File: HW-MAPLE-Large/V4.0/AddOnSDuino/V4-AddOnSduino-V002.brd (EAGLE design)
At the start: 31 x 22.1 mm, 5 parts

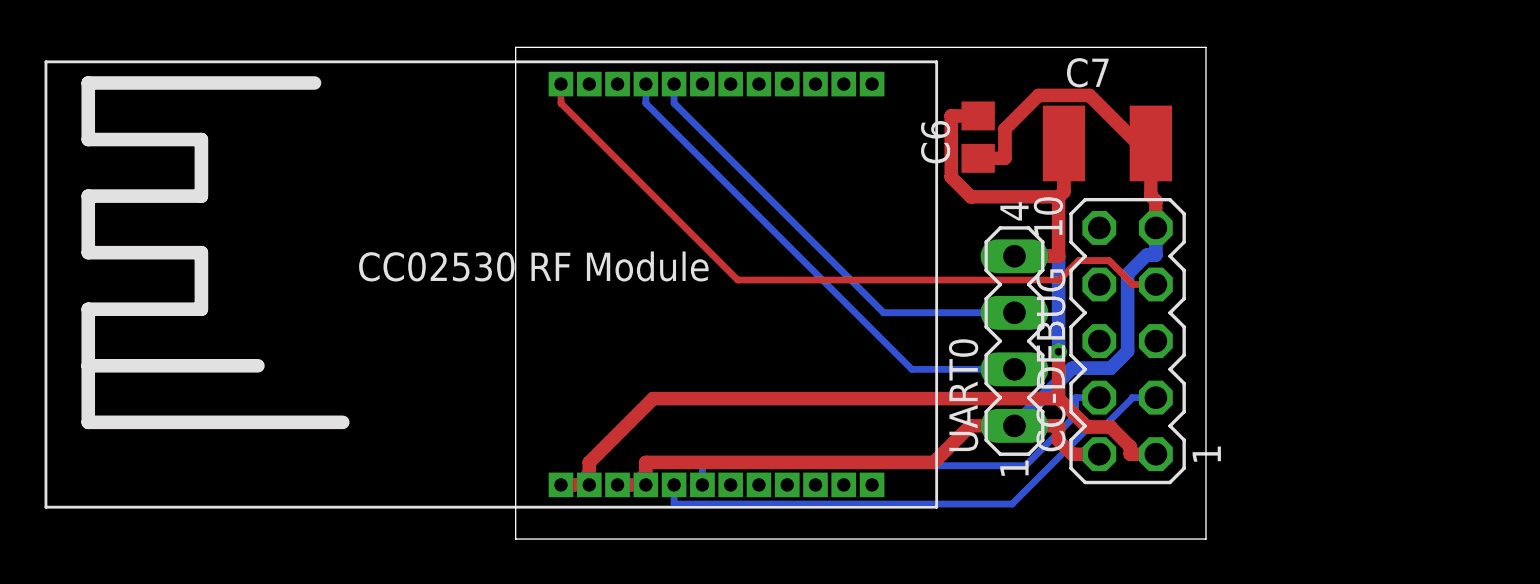
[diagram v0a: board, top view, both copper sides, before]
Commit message: V4 Test
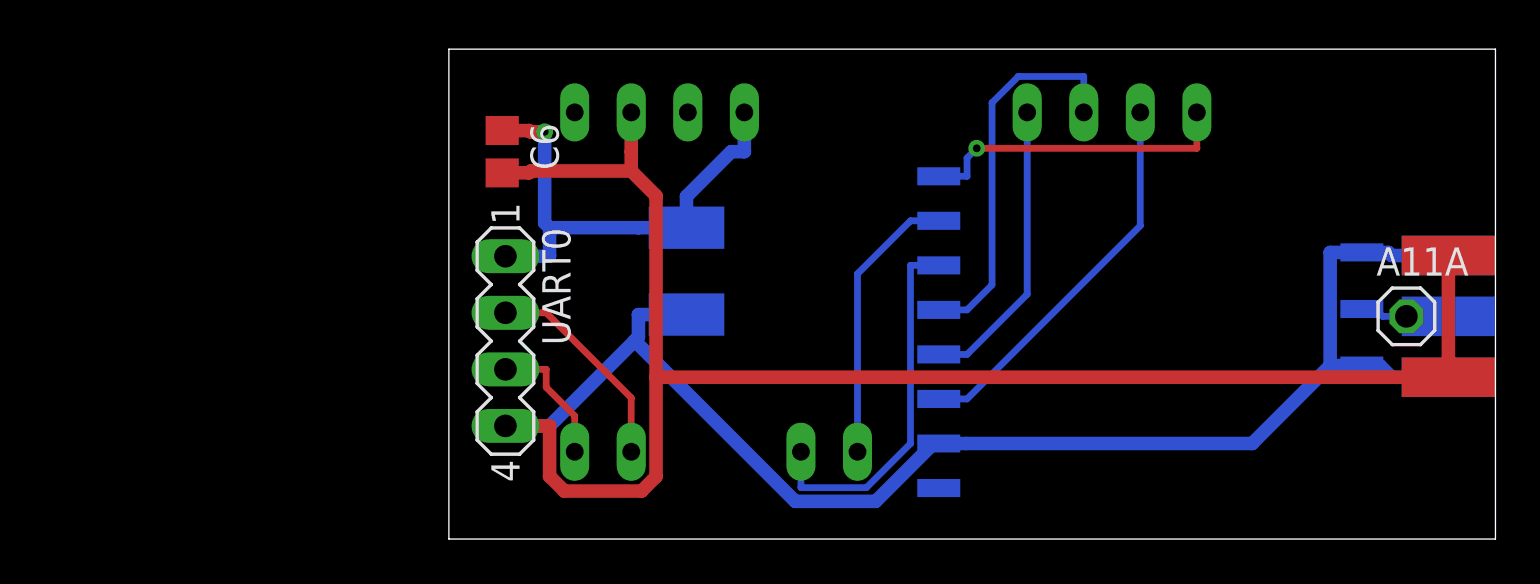
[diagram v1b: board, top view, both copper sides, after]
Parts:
- removed CC-DEBUG: (no value), con-lstb:MA05-2
- removed U$1: CC2530CC2530PA, zigbee:CC2530PA
- added A11A: (no value), pinhead:1X01
- added A11B: SMA, wireless:SMA
- added CC1101: CC1101_MODULE1SMD, CC1101:CC1101_MODULE1_SMD
- added U$2: MARTIN-PROMINI-CC1101, Arduino-clone:MARTIN-PRO-CC1101
- moved UART0 22.9 mm to (2.54, 8.89), turned to 270 degrees
- moved C6 21.4 mm to (2.40, 17.4), turned to 270 degrees
- moved C7 19.8 mm to (10.7, 12.0), flipped to the bottom, turned to 90 degrees
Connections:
- removed net BT: U$1.P$6
- removed net CS: CC-DEBUG.5
- removed net DC: CC-DEBUG.3, U$1.P$8
- removed net DD: CC-DEBUG.4, U$1.P$7
- removed net RST: CC-DEBUG.7, U$1.P$24
- removed net RX0: U$1.P$20, UART0.3
- removed net SCLK: CC-DEBUG.6
- removed net TX0: U$1.P$21, UART0.2
- new net +3V3: CC1101.VCC
- new net ANT1: A11A.1, A11B.1, CC1101.ANT
- new net CSN: CC1101.CSN, U$2.D10
- new net GDO0_D3: CC1101.GDO0, U$2.D3
- new net GDO2_D2: CC1101.GDO2, U$2.D2
- new net RX-MAPLE0: U$2.TX0, UART0.3
- new net SCK: CC1101.SCLK, U$2.D13
- new net TX-MAPLE0: U$2.RX1, UART0.2
- net GND: now also A11B.GND@1, A11B.GND@2, A11B.GND@3, A11B.GND@4, CC1101.GND@0, CC1101.GND@1, CC1101.GND@2, U$2.GND; no longer CC-DEBUG.1, U$1.P$11, U$1.P$12
- net MISO: now also CC1101.MISO, U$2.D12; no longer CC-DEBUG.10
- net MOSI: now also CC1101.MOSI, U$2.D11; no longer CC-DEBUG.8
- net VCC: now also U$2.VCC; no longer CC-DEBUG.2, CC-DEBUG.9, U$1.P$10, U$1.P$9
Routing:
- net GND: track 55.2 -> 136.8 mm, vias 1 -> 0
- net RST: track 31.7 -> 0.00 mm
- net VCC: track 52.6 -> 22.3 mm, vias 0 -> 1
- net DC: track 24.5 -> 0.00 mm
- net TX0: track 22.4 -> 0.00 mm
- net DD: track 20.4 -> 0.00 mm
- net RX0: track 20.0 -> 0.00 mm
- net MOSI: track 0.00 -> 17.4 mm
- net MISO: track 0.00 -> 17.3 mm
- net GDO2_D2: track 0.00 -> 16.6 mm
- net CSN: track 0.00 -> 14.2 mm, vias 0 -> 1
- net SCK: track 0.00 -> 13.3 mm
- net GDO0_D3: track 0.00 -> 12.6 mm
- net TX-MAPLE0: track 0.00 -> 9.65 mm
- net RX-MAPLE0: track 0.00 -> 6.06 mm
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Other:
- board size 31 x 22.1 mm -> 47 x 22 mm
